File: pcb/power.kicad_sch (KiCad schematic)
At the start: 14 parts, among them J5 Conn_01x04, Q1 BT148, U3 KA78M05_TO252

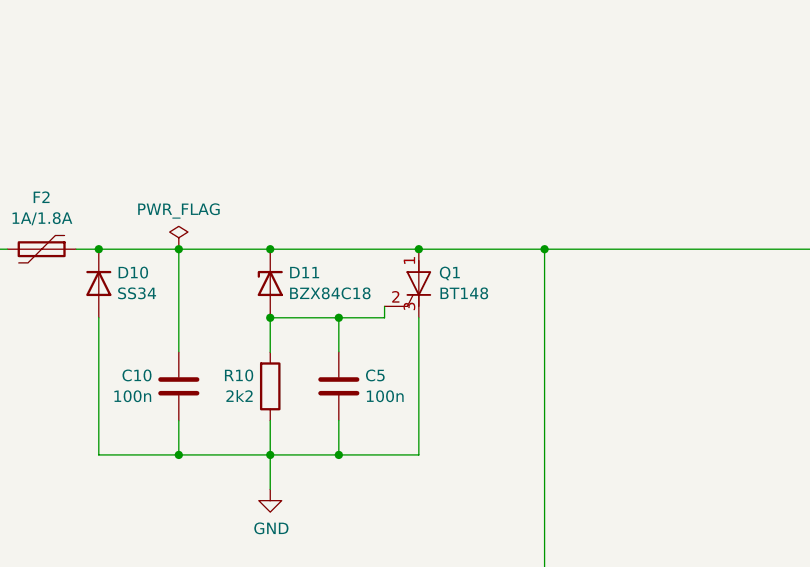
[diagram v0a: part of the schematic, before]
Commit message: Fix bad BT148 pinout & fix connected wires.
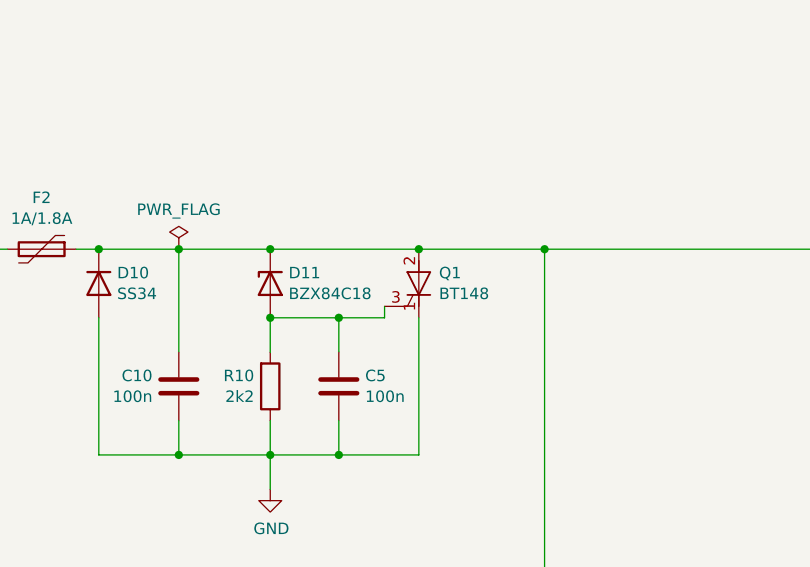
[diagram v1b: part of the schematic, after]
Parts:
- Q1: symbol Triac_Thyristor:BT169D -> Device:Q_SCR_KAG
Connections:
- net GND: now also Q1.1 (K); no longer Q1.3 (K)
- net STEPIN: now also Q1.2 (A); no longer Q1.1 (A)
- net at C5.1, D11.2 (A), R10.2: now also Q1.3 (G); no longer Q1.2 (G)
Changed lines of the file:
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@@
     (pin "2")
   )
-  (symbol (lib_id "Triac_Thyristor:BT169D") (at 86.36 63.5 0) (unit 1)
+  (symbol (lib_id "Device:Q_SCR_KAG") (at 86.36 63.5 0) (unit 1)
     (in_bom yes) (on_board yes)
     (property "Reference" "Q1" (id 0) (at 88.5952 62.3316 0)
@@
       (effects (font (size 1.27 1.27)) (justify left))
     )
-    (property "Footprint" "Package_TO_SOT_SMD:SOT-223" (id 2) (at 88.9 65.405 0)
-      (effects (font (size 1.27 1.27) italic) (justify left) hide)
+    (property "Footprint" "Package_TO_SOT_SMD:SOT-223" (id 2) (at 86.36 63.5 90)
+      (effects (font (size 1.27 1.27)) hide)
     )
-    (property "Datasheet" "https://media.digikey.com/pdf/Data%20Sheets/NXP%20PDFs/BT169_Series.pdf" (id 3) (at 86.36 63.5 0)
-      (effects (font (size 1.27 1.27)) (justify left) hide)
+    (property "Datasheet" "~" (id 3) (at 86.36 63.5 90)
+      (effects (font (size 1.27 1.27)) hide)
     )
     (property "LCSC" "C256433" (id 4) (at 86.36 63.5 0)

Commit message: Update libraries, add JLCPCB tooling holes.
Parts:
- D11: footprint Diode_SMD:D_SOT-23_ANK -> Package_TO_SOT_SMD:SOT-23; LCSC (none) -> C841166
- J5: JLCPCB_IGNORE (none) -> true
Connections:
- net STEPIN: now also D11.3 (K); no longer D11.1 (K)
- net at C5.1, Q1.3 (G), R10.2: now also D11.1 (A); no longer D11.2 (A)
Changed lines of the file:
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@@
   (symbol (lib_id "power:GND") (at 161.29 80.01 0) (unit 1)
     (in_bom yes) (on_board yes)
-    (property "Reference" "#PWR027" (id 0) (at 161.29 86.36 0)
+    (property "Reference" "#PWR0127" (id 0) (at 161.29 86.36 0)
       (effects (font (size 1.27 1.27)) hide)
     )
@@
       (effects (font (size 1.27 1.27)) (justify right))
     )
-    (property "Footprint" "Diode_SMD:D_SOT-23_ANK" (id 2) (at 74.295 63.5 0)
+    (property "Footprint" "Package_TO_SOT_SMD:SOT-23" (id 2) (at 74.295 63.5 0)
       (effects (font (size 1.27 1.27)) hide)
     )
@@
       (effects (font (size 1.27 1.27)) hide)
     )
-    (property "LCSC" "" (id 4) (at 69.85 63.5 0)
+    (property "LCSC" "C841166" (id 4) (at 69.85 63.5 0)
       (effects (font (size 1.27 1.27)) hide)
     )
@@
     (pin "1")
     (pin "2")
+    (pin "3")
   )
   (symbol (lib_id "power:VCC") (at 185.42 115.57 0) (unit 1)
     (in_bom yes) (on_board yes)
-    (property "Reference" "#PWR030" (id 0) (at 185.42 119.38 0)
+    (property "Reference" "#PWR016" (id 0) (at 185.42 119.38 0)
       (effects (font (size 1.27 1.27)) hide)
     )
@@
       (effects (font (size 1.27 1.27)) hide)
     )
+    (property "JLCPCB_IGNORE" "true" (id 4) (at 163.83 41.91 0)
+      (effects (font (size 1.27 1.27)) hide)
+    )
     (pin "1")
     (pin "2")
@@
   (symbol (lib_id "power:GND") (at 185.42 130.81 0) (unit 1)
     (in_bom yes) (on_board yes)
-    (property "Reference" "#PWR033" (id 0) (at 185.42 137.16 0)
+    (property "Reference" "#PWR0129" (id 0) (at 185.42 137.16 0)
       (effects (font (size 1.27 1.27)) hide)
     )
@@
   (symbol (lib_id "power:GND") (at 165.1 130.81 0) (unit 1)
     (in_bom yes) (on_board yes)
-    (property "Reference" "#PWR032" (id 0) (at 165.1 137.16 0)
+    (property "Reference" "#PWR0130" (id 0) (at 165.1 137.16 0)
       (effects (font (size 1.27 1.27)) hide)
     )
@@
   (symbol (lib_id "power:GND") (at 144.78 130.81 0) (unit 1)
     (in_bom yes) (on_board yes)
-    (property "Reference" "#PWR031" (id 0) (at 144.78 137.16 0)
+    (property "Reference" "#PWR0128" (id 0) (at 144.78 137.16 0)
       (effects (font (size 1.27 1.27)) hide)
     )
@@
   (symbol (lib_id "power:GND") (at 166.37 80.01 0) (unit 1)
     (in_bom yes) (on_board yes)
-    (property "Reference" "#PWR028" (id 0) (at 166.37 86.36 0)
+    (property "Reference" "#PWR0132" (id 0) (at 166.37 86.36 0)
       (effects (font (size 1.27 1.27)) hide)
     )
@@
   (symbol (lib_id "power:GND") (at 69.85 86.36 0) (unit 1)
     (in_bom yes) (on_board yes)
-    (property "Reference" "#PWR029" (id 0) (at 69.85 92.71 0)
-      (effects (font (size 1.27 1.27)) hide)
-    )
+    (property "Reference" "#PWR0131" (id 0) (at 69.85 92.71 0)
+      (effects (font (size 1.27 1.27)) hide)
+    )
